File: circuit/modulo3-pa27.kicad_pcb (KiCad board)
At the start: 2 copper layers, 105 x 47 mm, 48 parts, among them J1 CONN_01X02, J3 CONN_01X04, J4 JACK_MONO, J5 HOLE, J7 HOLE, SW1 bright, U1 OPA2134, U2 OPA2134, U3 TLE2426, U4 PWR_CONN

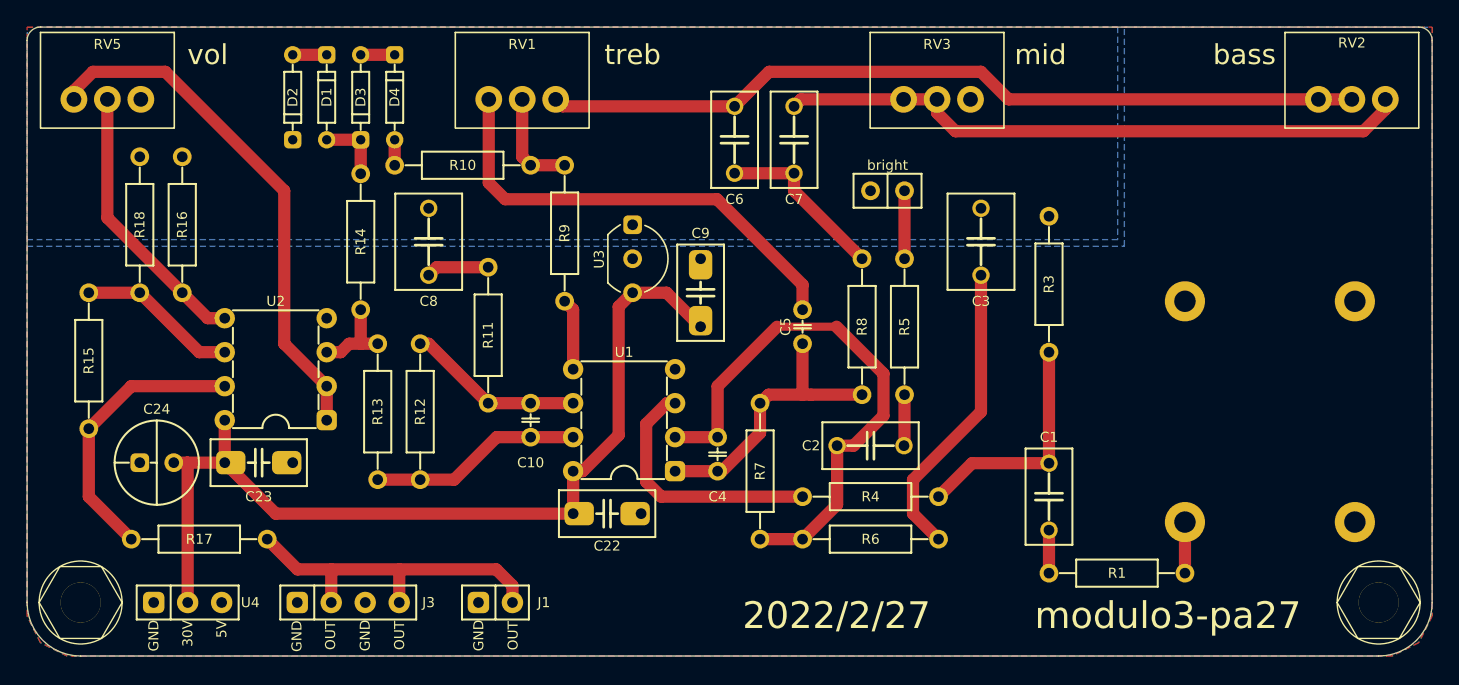
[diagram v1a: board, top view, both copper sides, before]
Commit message: ready to panelize
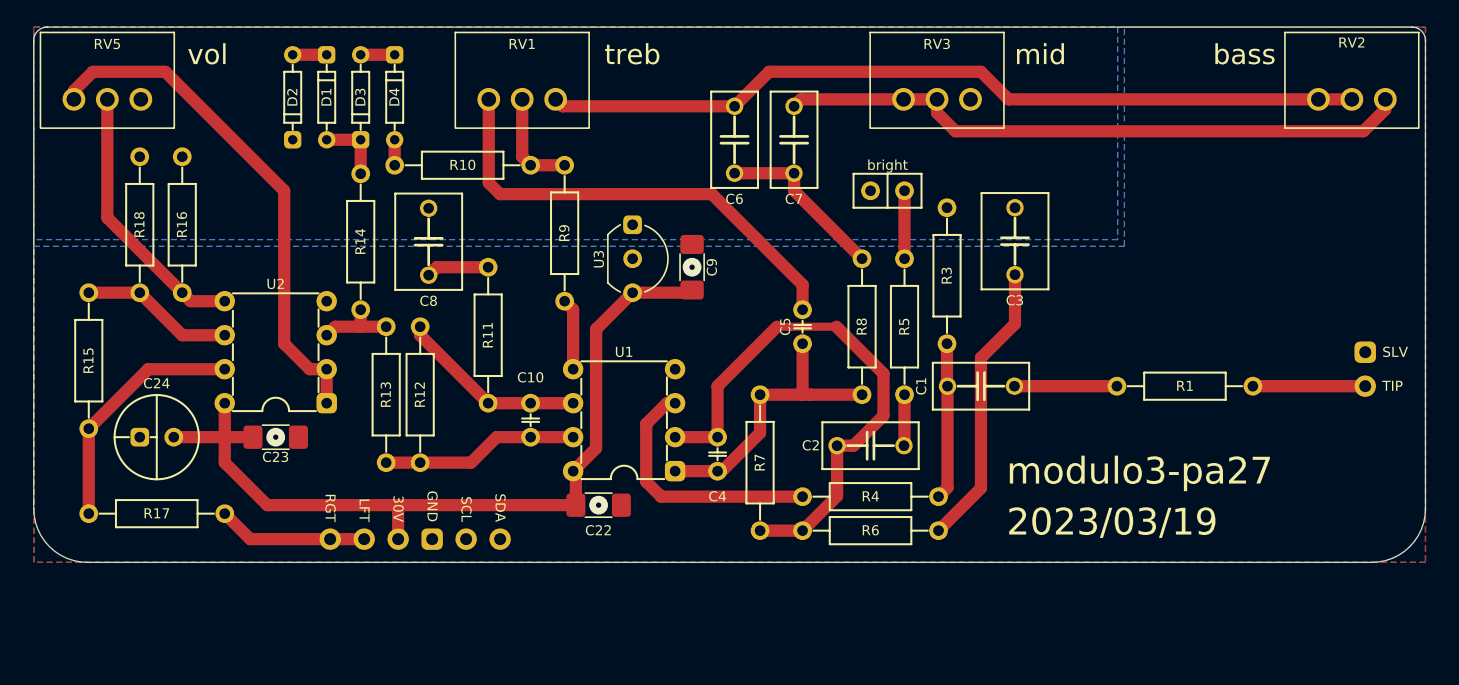
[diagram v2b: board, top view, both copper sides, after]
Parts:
- removed J1: CONN_01X02, myAmp:PIN_1x02
- removed J3: CONN_01X04, myAmp:PIN_1x04
- removed J4: JACK_MONO, myAmp:JACK_CL13106
- removed J5, J7: HOLE, myAmp:MountingHole
- added U5: ~, myAmp:PREAMP_CONN, F.Cu at (79.0, 88.3)
- C22, C23, C9: footprint myAmp:C_5MM_1206 -> myAmp:C_1206
- RV3: value B10k -> A10k
- U4: value PWR_CONN -> ~; footprint myAmp:PWR_CONN -> myAmp:EXT_JACK
- moved U4 90.0 mm to (150.0, 74.3)
- moved R1 14.9 mm to (136.5, 76.8)
- moved C1 9.69 mm to (121.3, 76.8), turned to 180 degrees
- moved R3 7.65 mm to (118.7, 68.6)
- moved R17 3.70 mm to (59.7, 86.4)
- moved C3 2.54 mm to (123.8, 66.0)
- moved C23 2.29 mm to (68.6, 80.6)
- moved C9 2.01 mm to (99.7, 67.9)
- moved C24 1.91 mm to (59.7, 80.6)
- moved R13 1.42 mm to (76.8, 77.5)
- moved R12 1.27 mm to (79.4, 77.5)
- moved U2 1.27 mm to (68.6, 74.3)
- moved C22 0.90 mm to (92.7, 85.7)
- moved R6 0.64 mm to (113.0, 87.6)
- moved R7 0.64 mm to (104.8, 82.5)
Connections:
- C22 pad 2: +24V -> +28V
- C23 pad 2: +24V -> +28V
- C24 pad 1: +24V -> +28V
- C9 pad 2: +24V -> +28V
- R1 pad 2: Net-(J4-Pad6) -> Net-(U4-TIP)
- U1 pad 8: +24V -> +28V
- U2 pad 8: +24V -> +28V
- U3 pad 3: +24V -> +28V
- U4 pad 2: +24V -> Net-(U4-TIP)
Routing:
- net +24V: track 70.0 -> 0.00 mm
- net +28V: track 0.00 -> 62.9 mm
- net /PA_OUT: track 26.0 -> 11.2 mm
- net Net-(U4-TIP): track 0.00 -> 8.40 mm
- net Net-(C1-Pad2): track 17.6 -> 11.7 mm
- net Net-(C1-Pad1): track 3.22 -> 7.66 mm
- net Net-(J4-Pad6): track 3.82 -> 0.00 mm
- net Net-(R15-Pad1): track 21.0 -> 18.4 mm
- net Net-(C10-Pad2): track 15.9 -> 14.8 mm
- net Net-(C3-Pad2): track 22.6 -> 21.5 mm
- net Net-(U1B--): track 13.3 -> 14.2 mm
- net Net-(U2A-+): track 6.61 -> 5.98 mm
- net Net-(U1A--): track 41.4 -> 40.8 mm
- net Net-(U2A--): track 39.1 -> 38.6 mm
- net Net-(U2B--): track 12.0 -> 11.5 mm
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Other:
- board size 105 x 47 mm -> 104 x 40 mm
- board text added: "2023/03/19"
- board text removed: "2022/2/27"
- board text removed: "GND"
- board text removed: "OUT"
